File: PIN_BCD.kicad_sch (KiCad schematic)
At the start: 16 parts, among them J10 Conn_01x06_MountingPin, J11 Conn_01x03_Pin, J12 Conn_01x04_MountingPin, J4 Conn_01x04_MountingPin, J5 Conn_01x03_Pin, J6 Conn_01x02_MountingPin, J7 Conn_01x06_MountingPin, J8 Conn_01x06_MountingPin, J9 Conn_01x06_MountingPin, Q2 SS8050, U1 HPM5E31IPB1, U13 AFA11-S08GLA-00

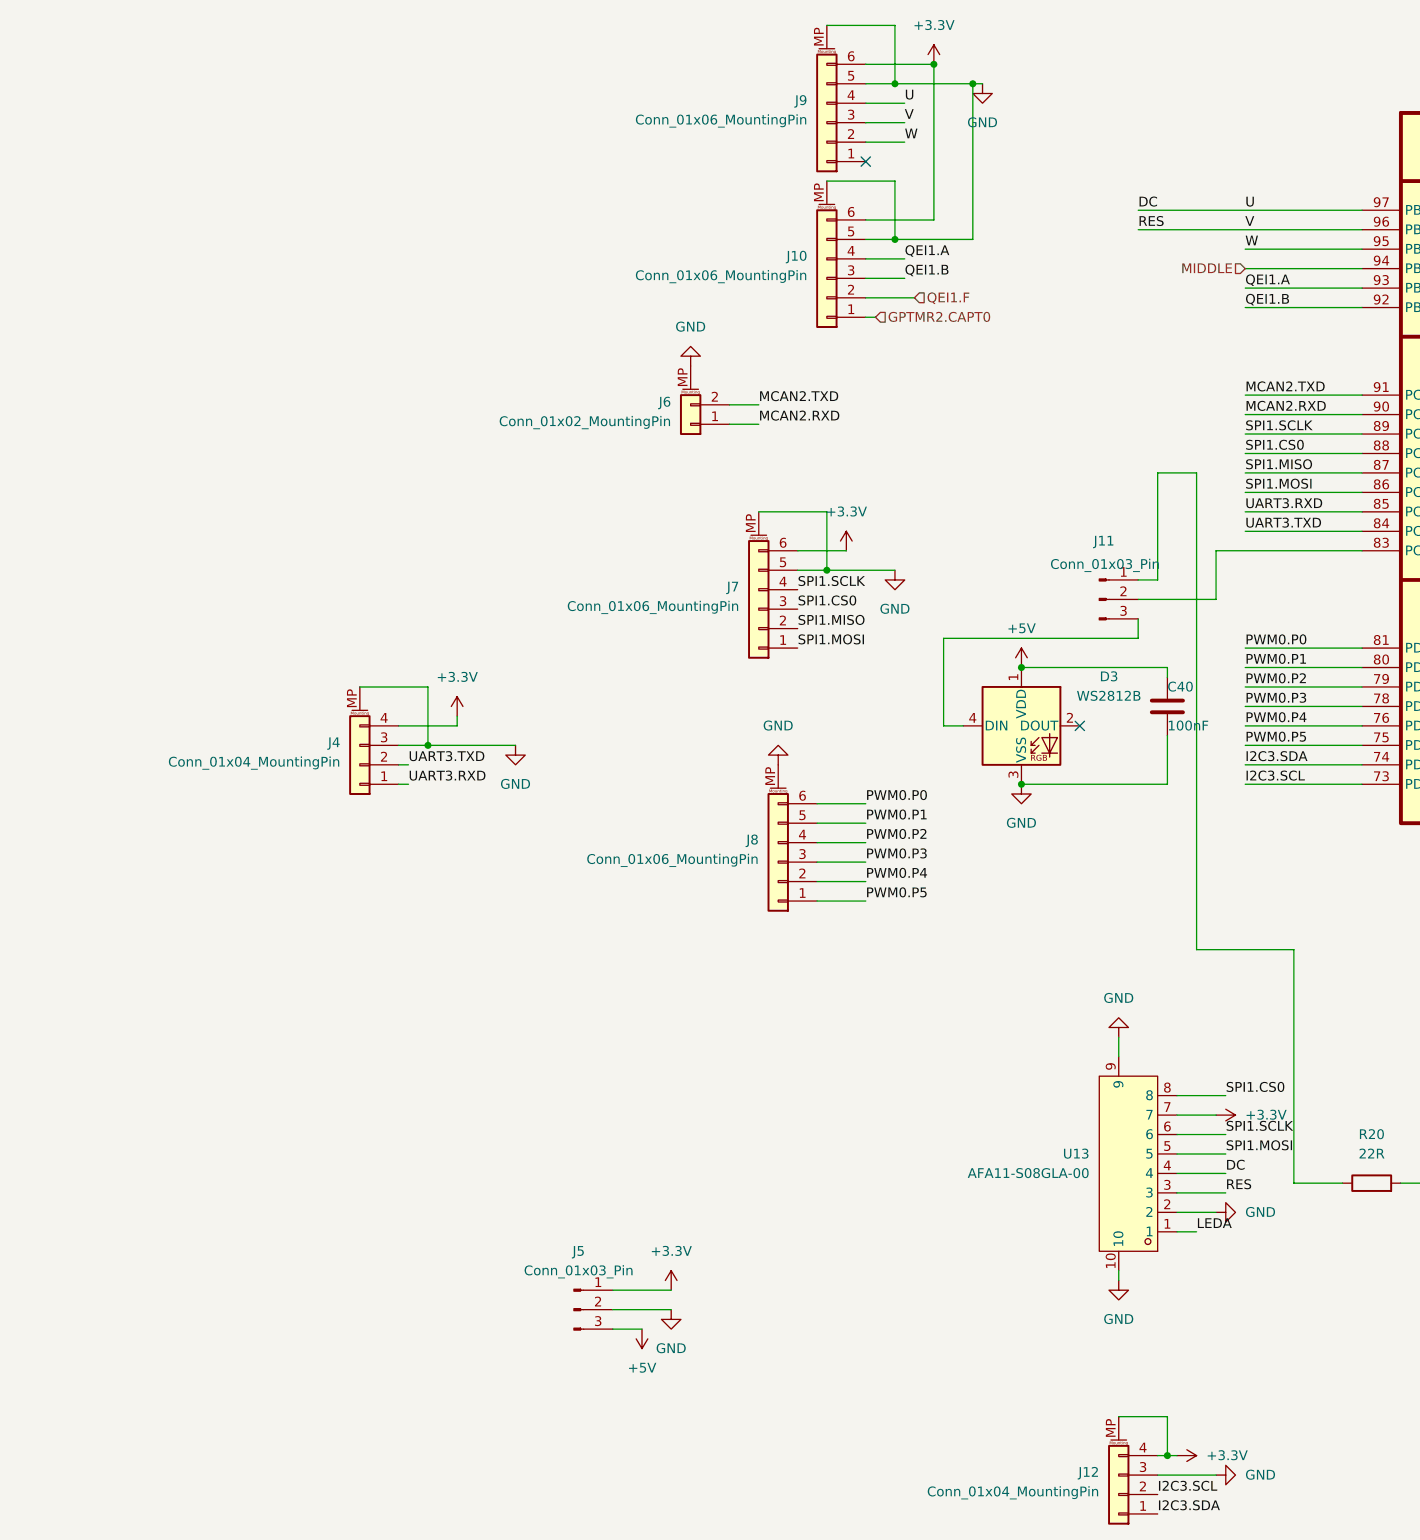
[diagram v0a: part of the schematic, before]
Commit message: finish
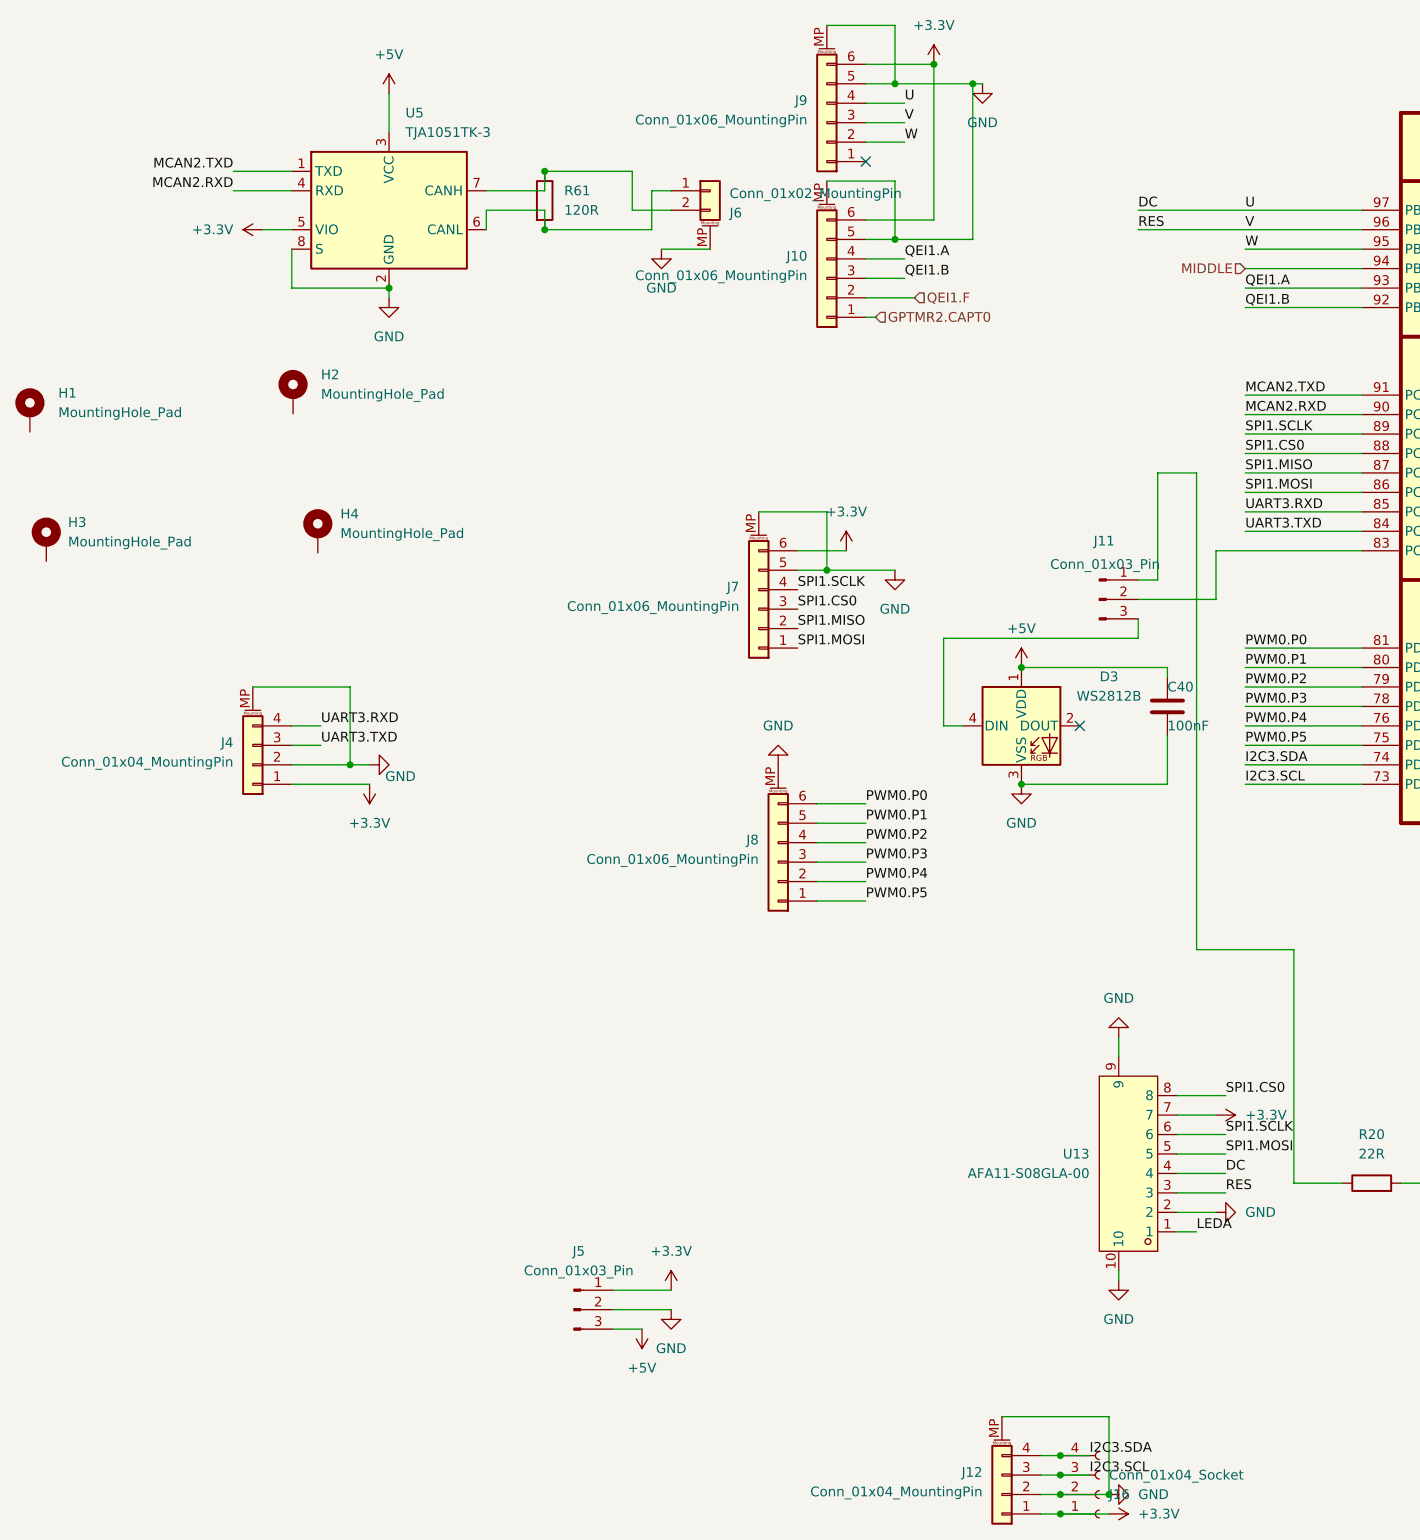
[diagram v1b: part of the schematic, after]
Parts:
- added H1, H2, H3, H4: MountingHole_Pad, MountingHole:MountingHole_2.2mm_M2_Pad, symbol Mechanical:MountingHole_Pad
- added J16: Conn_01x04_Socket, Connector_Harwin:Harwin_M20-89004xx_1x04_P2.54mm_Horizontal, symbol Connector:Conn_01x04_Socket
- added R61: 120R, Resistor_SMD:R_0603_1608Metric, symbol Device:R
- added U5: TJA1051TK-3, Package_SON:HVSON-8-1EP_3x3mm_P0.65mm_EP1.6x2.4mm, symbol Interface_CAN_LIN:TJA1051TK-3
- J5: footprint Connector_PinHeader_2.54mm:PinHeader_1x03_P2.54mm_Horizontal -> Connector_PinHeader_2.54mm:PinHeader_1x03_P2.54mm_Vertical
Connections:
- net +3.3V: now also J12.1 (Pin_1), J4.1 (Pin_1), J16.1 (Pin_1), U5.5 (VIO); no longer J12.4 (Pin_4), J12.MP (MountPin), J4.4 (Pin_4)
- net +5V: now also U5.3 (VCC)
- net GND: now also J12.2 (Pin_2), J12.MP (MountPin), J4.2 (Pin_2), J16.2 (Pin_2), U5.2 (GND), U5.8 (S), U5.9 (GND); no longer J12.3 (Pin_3), J4.3 (Pin_3)
- net I2C3.SCL: now also J12.3 (Pin_3), J16.3 (Pin_3); no longer J12.2 (Pin_2)
- net I2C3.SDA: now also J12.4 (Pin_4), J16.4 (Pin_4); no longer J12.1 (Pin_1)
- net MCAN2.RXD: now also U5.4 (RXD); no longer J6.1 (Pin_1)
- net MCAN2.TXD: now also U5.1 (TXD); no longer J6.2 (Pin_2)
- net UART3.RXD: now also J4.4 (Pin_4); no longer J4.1 (Pin_1)
- net UART3.TXD: now also J4.3 (Pin_3); no longer J4.2 (Pin_2)
- new net: J6.2 (Pin_2), R61.1, U5.7 (CANH)
- new net: J6.1 (Pin_1), R61.2, U5.6 (CANL)
